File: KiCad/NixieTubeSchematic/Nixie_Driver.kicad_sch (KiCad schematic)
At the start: 24 parts

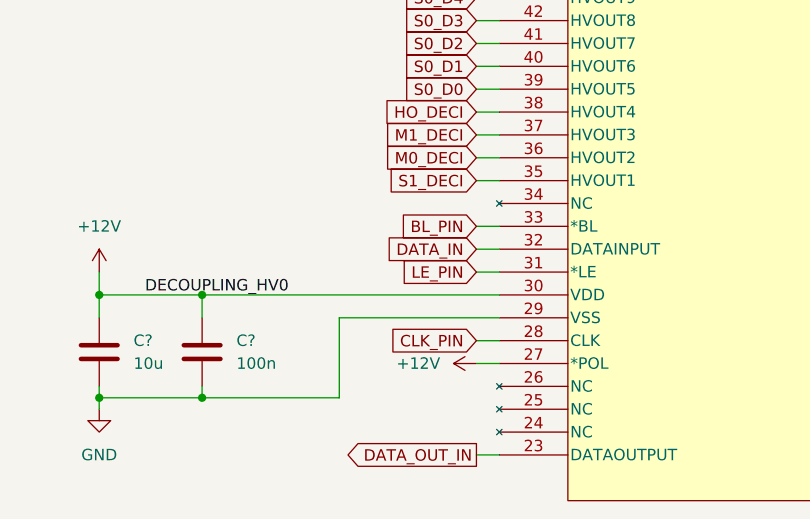
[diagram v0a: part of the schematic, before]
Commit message: Small changes
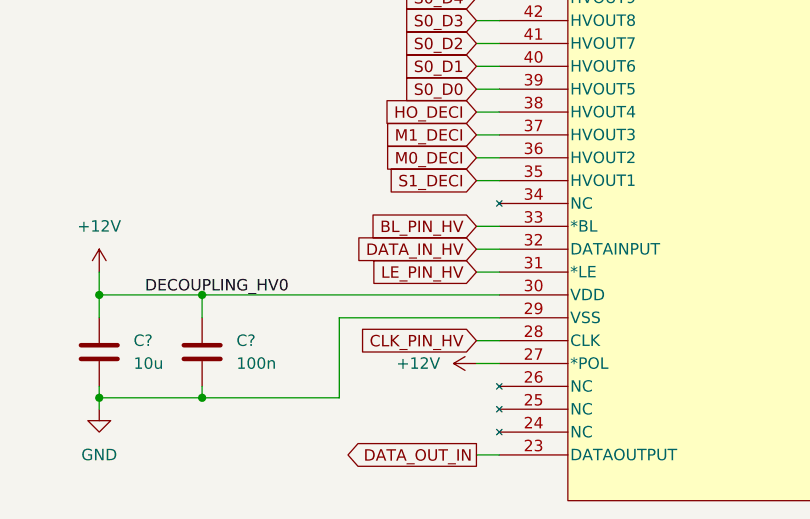
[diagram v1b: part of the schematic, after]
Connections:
- net BL_PIN: no longer U?.33 (*BL)
- net CLK_PIN: no longer U?.28 (CLK)
- net LE_PIN: no longer U?.31 (*LE)
- net DATA_IN renamed DATA_IN_HV
- new net BL_PIN_HV: U?.33 (*BL)
- new net CLK_PIN_HV: U?.28 (CLK)
- new net LE_PIN_HV: U?.31 (*LE)
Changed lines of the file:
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@@
     )
   )
-  (global_label "DATA_IN" (shape input) (at 67.31 133.35 180) (fields_autoplaced)
-    (effects (font (size 1.27 1.27)) (justify right))
-    (property "Intersheetrefs" "${INTERSHEET_REFS}" (at 57.5793 133.2706 0)
+  (global_label "DATA_IN_HV" (shape input) (at 67.31 133.35 180) (fields_autoplaced)
+    (effects (font (size 1.27 1.27)) (justify right))
+    (property "Intersheetrefs" "${INTERSHEET_REFS}" (at 53.6998 133.35 0)
       (effects (font (size 1.27 1.27)) (justify right) hide)
     )
@@
     )
   )
-  (global_label "BL_PIN" (shape input) (at 67.31 130.81 180) (fields_autoplaced)
-    (effects (font (size 1.27 1.27)) (justify right))
-    (property "Intersheetrefs" "${INTERSHEET_REFS}" (at 58.4259 130.7306 0)
+  (global_label "BL_PIN_HV" (shape input) (at 67.31 130.81 180) (fields_autoplaced)
+    (effects (font (size 1.27 1.27)) (justify right))
+    (property "Intersheetrefs" "${INTERSHEET_REFS}" (at 54.5465 130.81 0)
       (effects (font (size 1.27 1.27)) (justify right) hide)
     )
@@
     )
   )
-  (global_label "LE_PIN" (shape input) (at 67.31 135.89 180) (fields_autoplaced)
-    (effects (font (size 1.27 1.27)) (justify right))
-    (property "Intersheetrefs" "${INTERSHEET_REFS}" (at 58.5469 135.8106 0)
+  (global_label "LE_PIN_HV" (shape input) (at 67.31 135.89 180) (fields_autoplaced)
+    (effects (font (size 1.27 1.27)) (justify right))
+    (property "Intersheetrefs" "${INTERSHEET_REFS}" (at 54.6675 135.89 0)
       (effects (font (size 1.27 1.27)) (justify right) hide)
     )
@@
     )
   )
-  (global_label "CLK_PIN" (shape input) (at 67.31 143.51 180) (fields_autoplaced)
-    (effects (font (size 1.27 1.27)) (justify right))
-    (property "Intersheetrefs" "${INTERSHEET_REFS}" (at 57.1559 143.4306 0)
-      (effects (font (size 1.27 1.27)) (justify right) hide)
-    )
+  (global_label "CLK_PIN_HV" (shape input) (at 67.31 143.51 180) (fields_autoplaced)
+    (effects (font (size 1.27 1.27)) (justify right))
+    (property "Intersheetrefs" "${INTERSHEET_REFS}" (at 53.2765 143.51 0)
+      (effects (font (size 1.27 1.27)) (justify right) hide)
+    )
